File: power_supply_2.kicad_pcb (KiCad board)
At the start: 2 copper layers, 106.7 x 43.2 mm, 42 parts, among them U1 LM317, U2 LM337

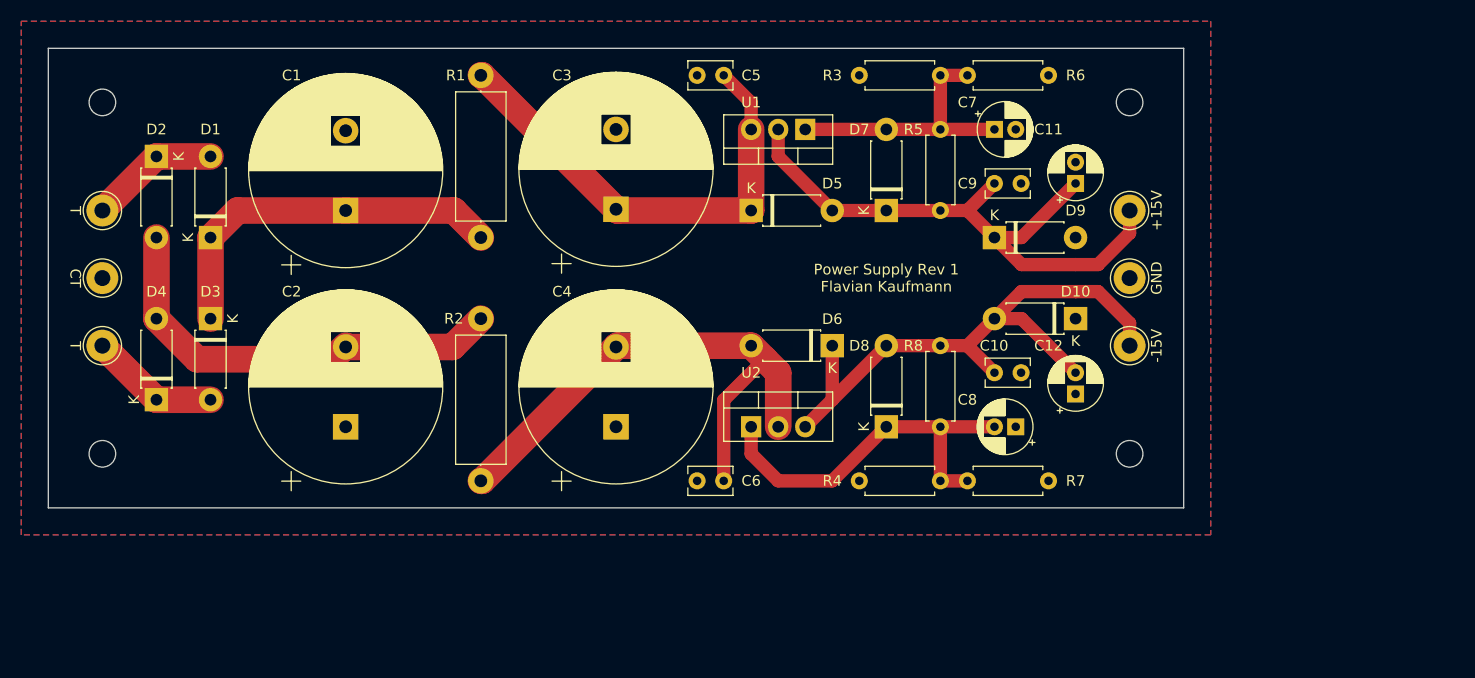
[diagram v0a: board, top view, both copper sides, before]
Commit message: cosmetics
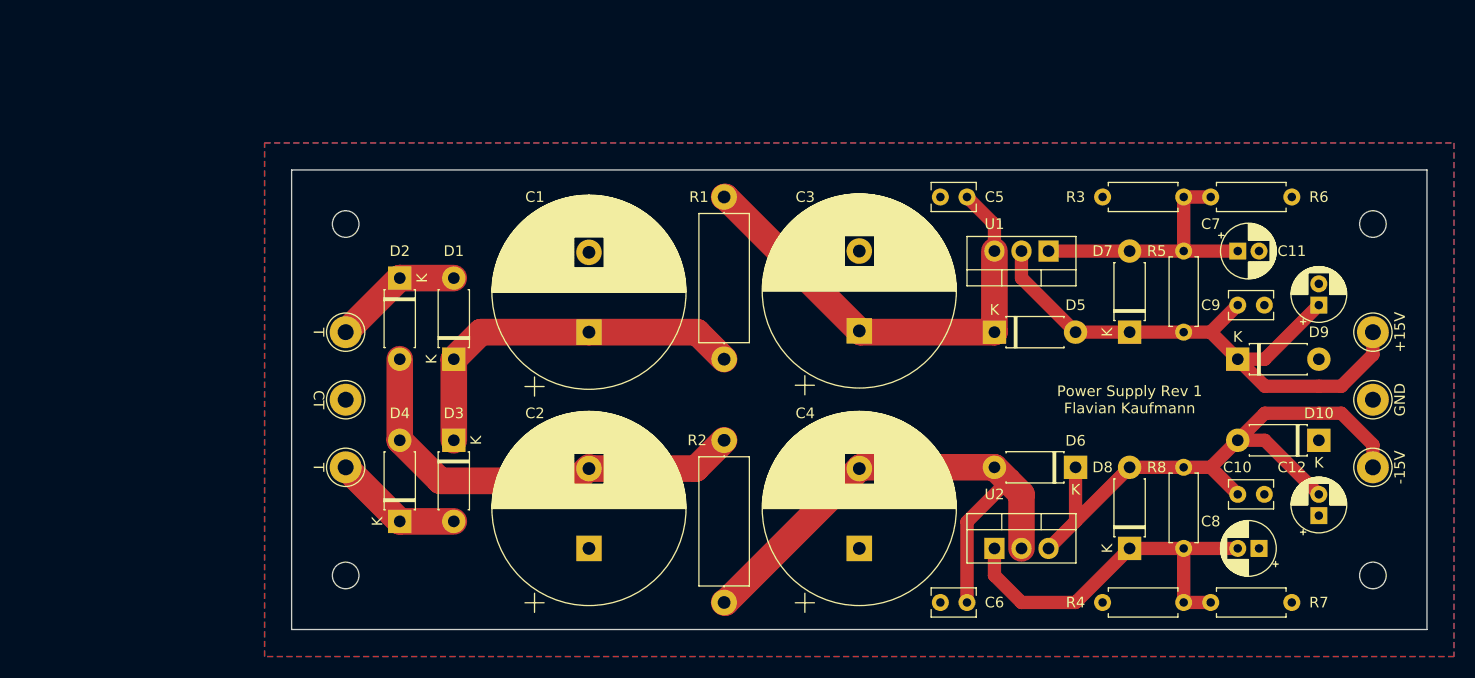
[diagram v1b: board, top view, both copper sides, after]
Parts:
- moved C3 25.6 mm to (142.2, 102.8)
- moved C5 25.6 mm to (152.4, 90.2)
- moved C6 25.6 mm to (149.9, 128.3)
- moved C7 25.6 mm to (177.8, 95.2)
- moved REF** 25.6 mm to (190.5, 102.9)
- moved REF** 25.6 mm to (190.5, 125.7)
- moved U1 25.6 mm to (160.0, 95.2)
- moved C1 25.6 mm to (116.8, 102.9)
- moved C10 25.6 mm to (180.3, 118.1)
- moved C4 25.6 mm to (142.2, 123.2)
- moved C8 25.6 mm to (179.8, 123.2)
- moved C9 25.6 mm to (177.8, 100.3)
- moved D2 25.6 mm to (99.1, 97.8)
- moved D3 25.6 mm to (104.1, 113.0)
- moved D4 25.6 mm to (99.1, 120.7)
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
